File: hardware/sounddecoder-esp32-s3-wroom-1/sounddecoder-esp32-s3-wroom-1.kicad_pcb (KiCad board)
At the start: 2 copper layers, 16 parts, among them J5 UART, U1 LM2596S-5, U2 IS25WP256D-xM, U3 MAX98357A, U4 DRV8871DDA, U6 AMS1117-3.3, U7 ESP32-S3-WROOM-1

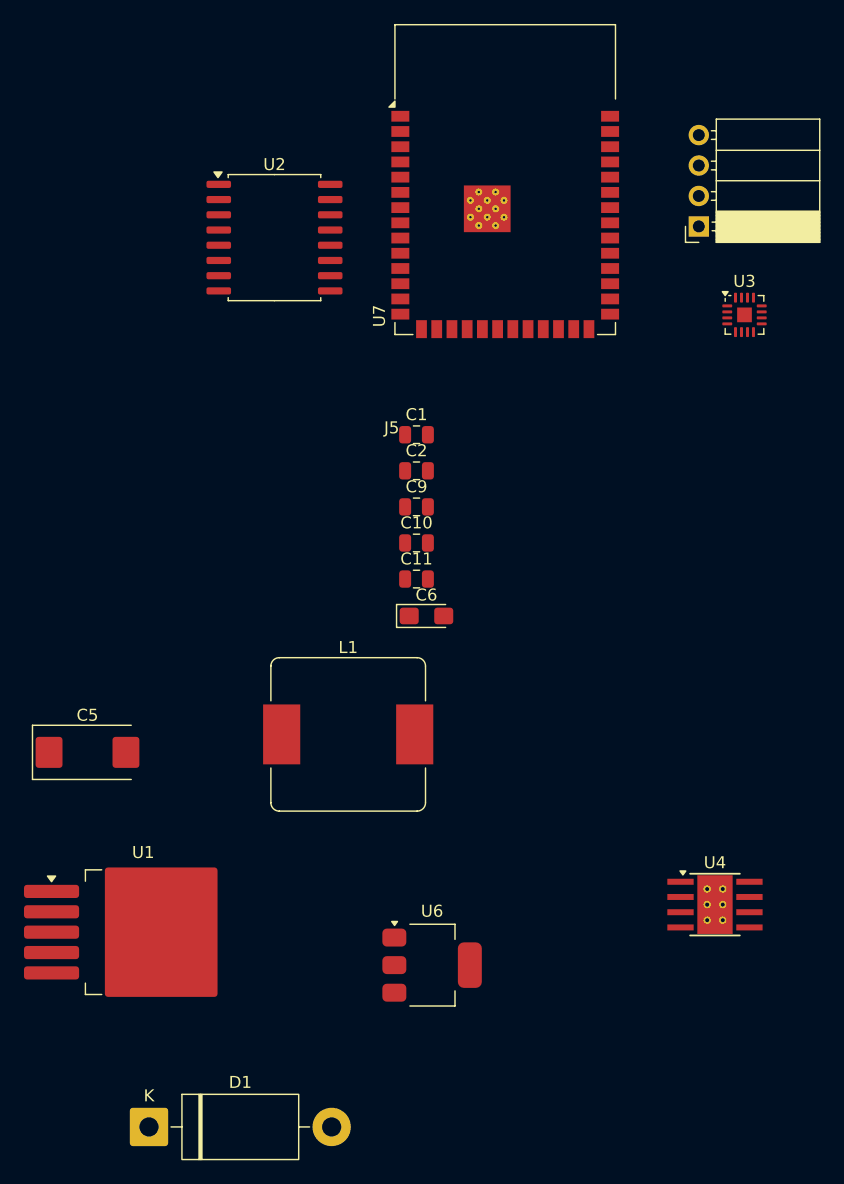
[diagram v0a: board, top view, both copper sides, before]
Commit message: Created PCB
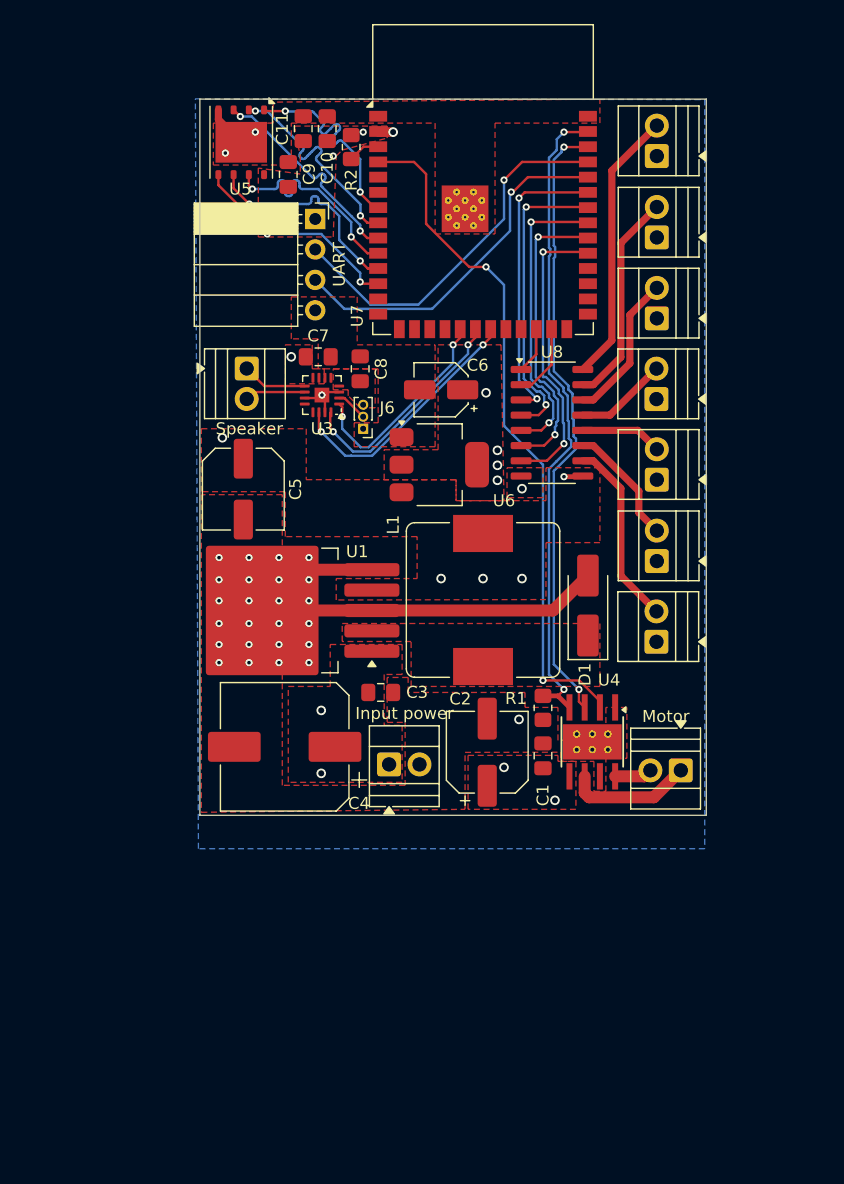
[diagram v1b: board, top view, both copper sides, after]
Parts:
- removed U2: IS25WP256D-xM, Package_SO:SOIC-16W_7.5x10.3mm_P1.27mm
- added C3: 0.1uF, Capacitor_SMD:C_0805_2012Metric_Pad1.18x1.45mm_HandSolder, F.Cu at (87.5, 125.5)
- added C4: 470uF, Capacitor_SMD:CP_Elec_10x10.5, F.Cu at (79.5, 130.0)
- added C7: 10uF, Capacitor_SMD:C_0805_2012Metric_Pad1.18x1.45mm_HandSolder, F.Cu at (82.2, 97.5)
- added C8: 0.1uF, Capacitor_SMD:C_0805_2012Metric_Pad1.18x1.45mm_HandSolder, F.Cu at (85.8, 98.5)
- added J1: Input power, TerminalBlock:TerminalBlock_Xinya_XY308-2.54-2P_1x02_P2.54mm_Horizontal, F.Cu at (88.2, 131.5)
- added J10: AUX1, TerminalBlock:TerminalBlock_Xinya_XY308-2.54-2P_1x02_P2.54mm_Horizontal, F.Cu at (110.5, 101.0)
- added J11: AUX2, TerminalBlock:TerminalBlock_Xinya_XY308-2.54-2P_1x02_P2.54mm_Horizontal, F.Cu at (110.5, 107.8)
- added J12: AUX3, TerminalBlock:TerminalBlock_Xinya_XY308-2.54-2P_1x02_P2.54mm_Horizontal, F.Cu at (110.5, 114.5)
- added J13: AUX4, TerminalBlock:TerminalBlock_Xinya_XY308-2.54-2P_1x02_P2.54mm_Horizontal, F.Cu at (110.5, 121.3)
- added J3: Motor, TerminalBlock:TerminalBlock_Xinya_XY308-2.54-2P_1x02_P2.54mm_Horizontal, F.Cu at (112.5, 132.0)
- added J4: Speaker, TerminalBlock:TerminalBlock_Xinya_XY308-2.54-2P_1x02_P2.54mm_Horizontal, F.Cu at (76.3, 98.5)
- added J6: Conn_01x03_Pin, Connector_PinHeader_1.00mm:PinHeader_1x03_P1.00mm_Vertical, F.Cu at (86.0, 103.5)
- added J7: Smoke, TerminalBlock:TerminalBlock_Xinya_XY308-2.54-2P_1x02_P2.54mm_Horizontal, F.Cu at (110.5, 80.8)
- added J8: FwdLED, TerminalBlock:TerminalBlock_Xinya_XY308-2.54-2P_1x02_P2.54mm_Horizontal, F.Cu at (110.5, 87.5)
- added J9: BackLED, TerminalBlock:TerminalBlock_Xinya_XY308-2.54-2P_1x02_P2.54mm_Horizontal, F.Cu at (110.5, 94.3)
- added R1: 15k, Resistor_SMD:R_0805_2012Metric_Pad1.20x1.40mm_HandSolder, F.Cu at (101.0, 126.8)
- added R2: 10k, Resistor_SMD:R_0805_2012Metric_Pad1.20x1.40mm_HandSolder, F.Cu at (85.0, 80.0)
- added U5: W25Q256, Package_SON:WSON-8-1EP_6x5mm_P1.27mm_EP3.4x4.3mm, F.Cu at (75.8, 79.6)
- added U8: ULN2003A, Package_SO:SO-16_3.9x9.9mm_P1.27mm, F.Cu at (101.8, 103.0)
- C1, C10, C11, C9: footprint Capacitor_SMD:C_0805_2012Metric -> Capacitor_SMD:C_0805_2012Metric_Pad1.18x1.45mm_HandSolder
- C2: footprint Capacitor_SMD:C_0805_2012Metric -> Capacitor_SMD:CP_Elec_6.3x5.4
- C5: footprint Capacitor_Tantalum_SMD:CP_EIA-7343-20_Kemet-V_HandSolder -> Capacitor_SMD:C_Elec_6.3x7.7
- C6: footprint Capacitor_Tantalum_SMD:CP_EIA-3216-10_Kemet-I_HandSolder -> Capacitor_SMD:CP_Elec_4x5.4
- D1: value 1N5825 -> SS54; footprint Diode_THT:D_DO-201AD_P15.24mm_Horizontal -> Diode_SMD:D_SMA_Handsoldering
- moved D1 56.9 mm to (104.8, 118.2), turned to 90 degrees
- moved U6 41.8 mm to (92.3, 106.5)
- moved C11 38.7 mm to (81.0, 78.5), turned to 90 degrees
- moved U3 35.9 mm to (82.6, 100.7), turned to 180 degrees
- moved C10 35.4 mm to (83.0, 78.5), turned to 90 degrees
- moved J5 32.0 mm to (82.0, 86.0), turned to 0 degrees
- moved C9 29.7 mm to (79.8, 82.3), turned to 90 degrees
- moved U1 29.2 mm to (79.1, 118.7), turned to 180 degrees
- moved C1 28.8 mm to (101.0, 130.8), turned to 90 degrees
- moved C5 25.5 mm to (76.0, 108.5), turned to -90 degrees
- moved C2 24.2 mm to (96.3, 130.5), turned to 90 degrees
- moved C6 18.9 mm to (92.5, 100.2), turned to 180 degrees
- moved U4 17.0 mm to (105.1, 129.6), turned to -90 degrees
- moved L1 15.9 mm to (96.0, 117.8), turned to 90 degrees
- moved U7 1.85 mm to (96.0, 82.7)
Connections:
- net Net-(D1-K) renamed /Out5V
- net Net-(J5-Pin_2) renamed /UART-TX
- net Net-(J5-Pin_3) renamed /UART-RX
- U3 pad 10: Net-(J4-Pin_2) -> /Sound2
- U3 pad 2: GND -> /SND_GAIN
- U3 pad 9: Net-(J4-Pin_1) -> /Sound1
- U4 pad 6: Net-(J3-Pin_1) -> /MOTOR1
- U4 pad 8: Net-(J3-Pin_2) -> /MOTOR2
- U7 pad 10: unconnected-(U7-IO17-Pad10) -> /MEM_IO3
- U7 pad 11: unconnected-(U7-IO18-Pad11) -> /MEM_SCK
- U7 pad 12: Net-(U2-~{CE}) -> /MEM_IO0
- U7 pad 17: Net-(U2-~{WP}/IO2) -> unconnected-(U7-IO9-Pad17)
- U7 pad 18: Net-(U2-~{HOLD}/IO3) -> unconnected-(U7-IO10-Pad18)
- U7 pad 5: Net-(U2-SI/IO0) -> unconnected-(U7-IO5-Pad5)
- U7 pad 6: Net-(U2-SO/IO1) -> unconnected-(U7-IO6-Pad6)
- U7 pad 7: Net-(U2-SCK) -> /MEM_CE
- U7 pad 8: unconnected-(U7-IO15-Pad8) -> /MEM_IO1
- U7 pad 9: unconnected-(U7-IO16-Pad9) -> /MEM_IO2
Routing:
- net Net-(U4-IN2): track 0.00 -> 57.5 mm, vias 0 -> 2
- net /MOTOR_SENSE: track 0.00 -> 54.5 mm, vias 0 -> 2
- net Net-(U4-IN1): track 0.00 -> 51.8 mm, vias 0 -> 2
- net GND: track 0.00 -> 50.2 mm, vias 0 -> 29
- net /UART-TX: track 0.00 -> 31.5 mm, vias 0 -> 1
- net /UART-RX: track 0.00 -> 30.1 mm, vias 0 -> 1
- net Net-(U7-IO40): track 0.00 -> 25.2 mm, vias 0 -> 2
- net Net-(U7-IO39): track 0.00 -> 25.0 mm, vias 0 -> 2
- net Net-(U7-IO41): track 0.00 -> 24.9 mm, vias 0 -> 2
- net Net-(U7-IO38): track 0.00 -> 24.8 mm, vias 0 -> 2
- net Net-(U7-IO42): track 0.00 -> 24.7 mm, vias 0 -> 2
- net /Smoke: track 0.00 -> 22.9 mm
- net Net-(U3-LRCLK): track 0.00 -> 21.4 mm, vias 0 -> 2
- net Net-(U3-BCLK): track 0.00 -> 19.4 mm, vias 0 -> 2
- net /MEM_CE: track 0.00 -> 18.1 mm, vias 0 -> 2
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- added copper zone on F.Cu, net +3.3V
- added copper zone on In2.Cu, net +3.3V
- added copper zone on F.Cu, net +5V
- added copper zone on In2.Cu, net +5V
- added copper zone on F.Cu, net /Out5V
- added copper zone on B.Cu, net GND
- added copper zone on F.Cu, net GND
- added copper zone on In1.Cu, net GND
- added copper zone on F.Cu, net VCC
- added copper zone on In2.Cu, net VCC
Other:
- board outline added: 42.2 x 59.8 mm
- copper layers 2 -> 4
- board text added: "+"
- board text added: "-"
- board text added: "AUX1"
- board text added: "AUX2"
- board text added: "AUX3"
- board text added: "AUX4"
- board text added: "BackLED"
- board text added: "FwdLED"
- board text added: "Smoke"
